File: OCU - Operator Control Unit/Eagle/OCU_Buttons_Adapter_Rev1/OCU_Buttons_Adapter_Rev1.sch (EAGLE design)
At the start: 10 parts, among them J1 1053091202, J2 1053091202, J3 1053091202, J4 1053091202, J5 505567-0271, J6 505567-0271, J7 505567-0371

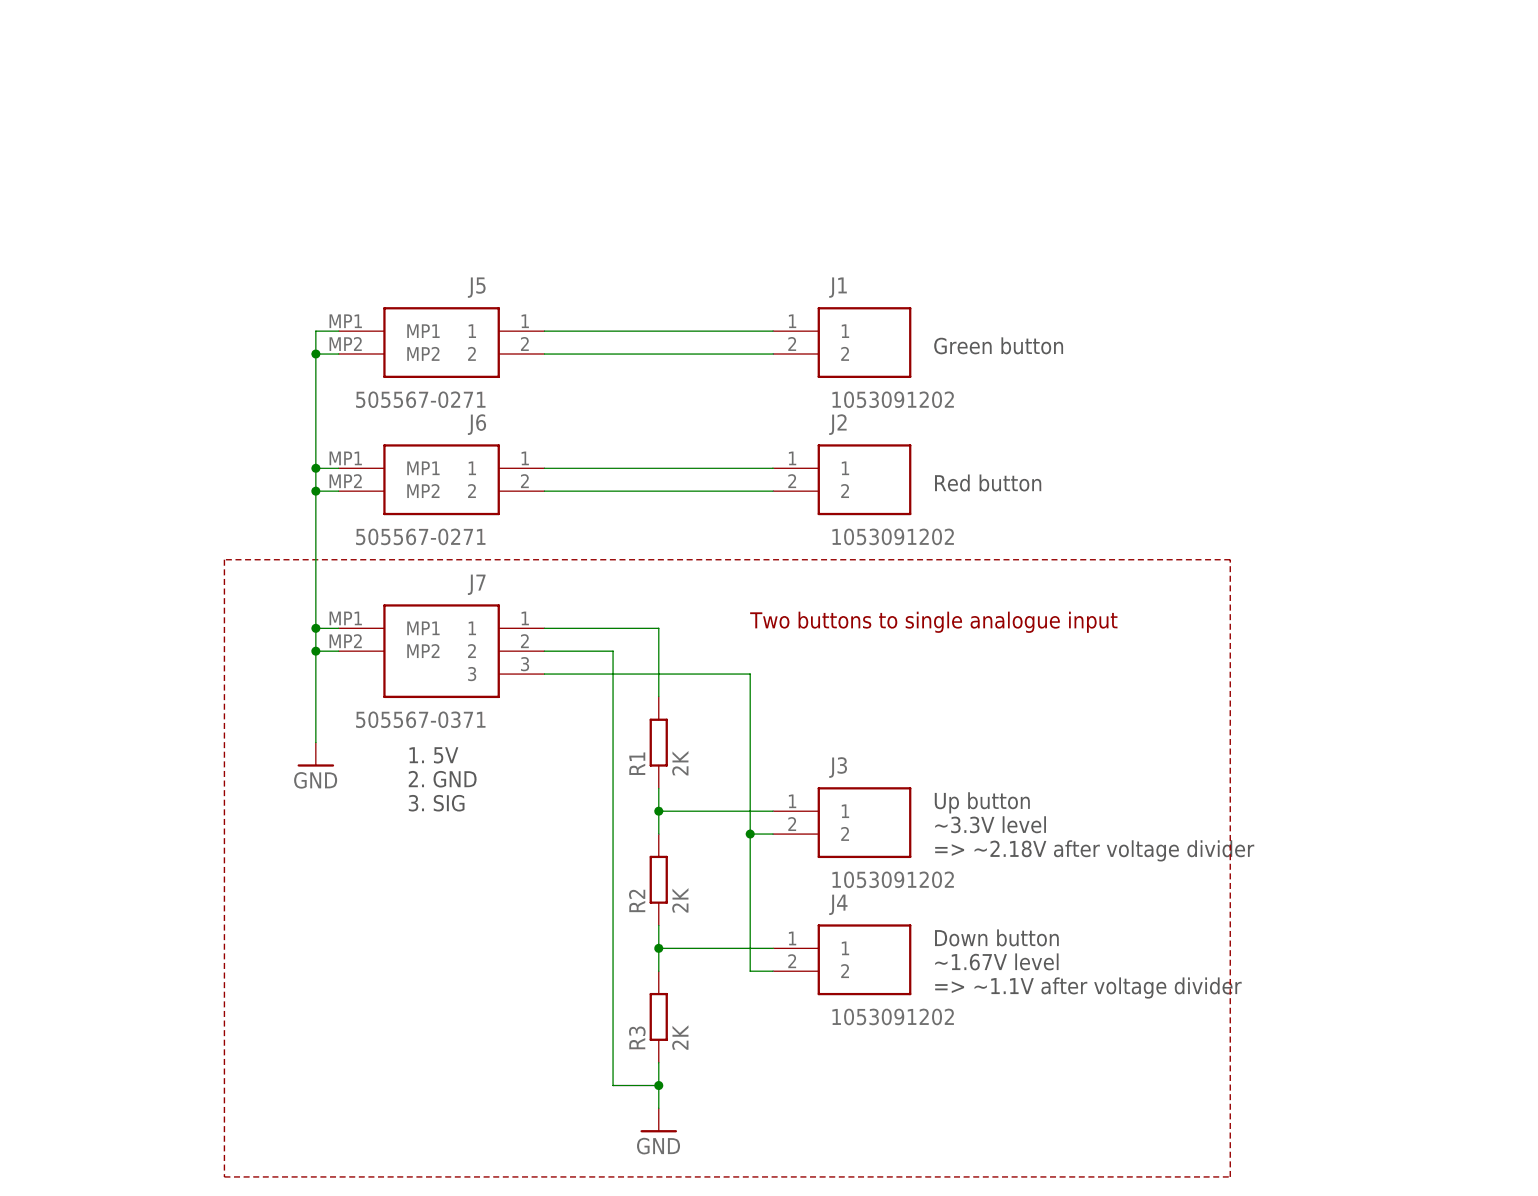
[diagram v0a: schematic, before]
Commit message: -
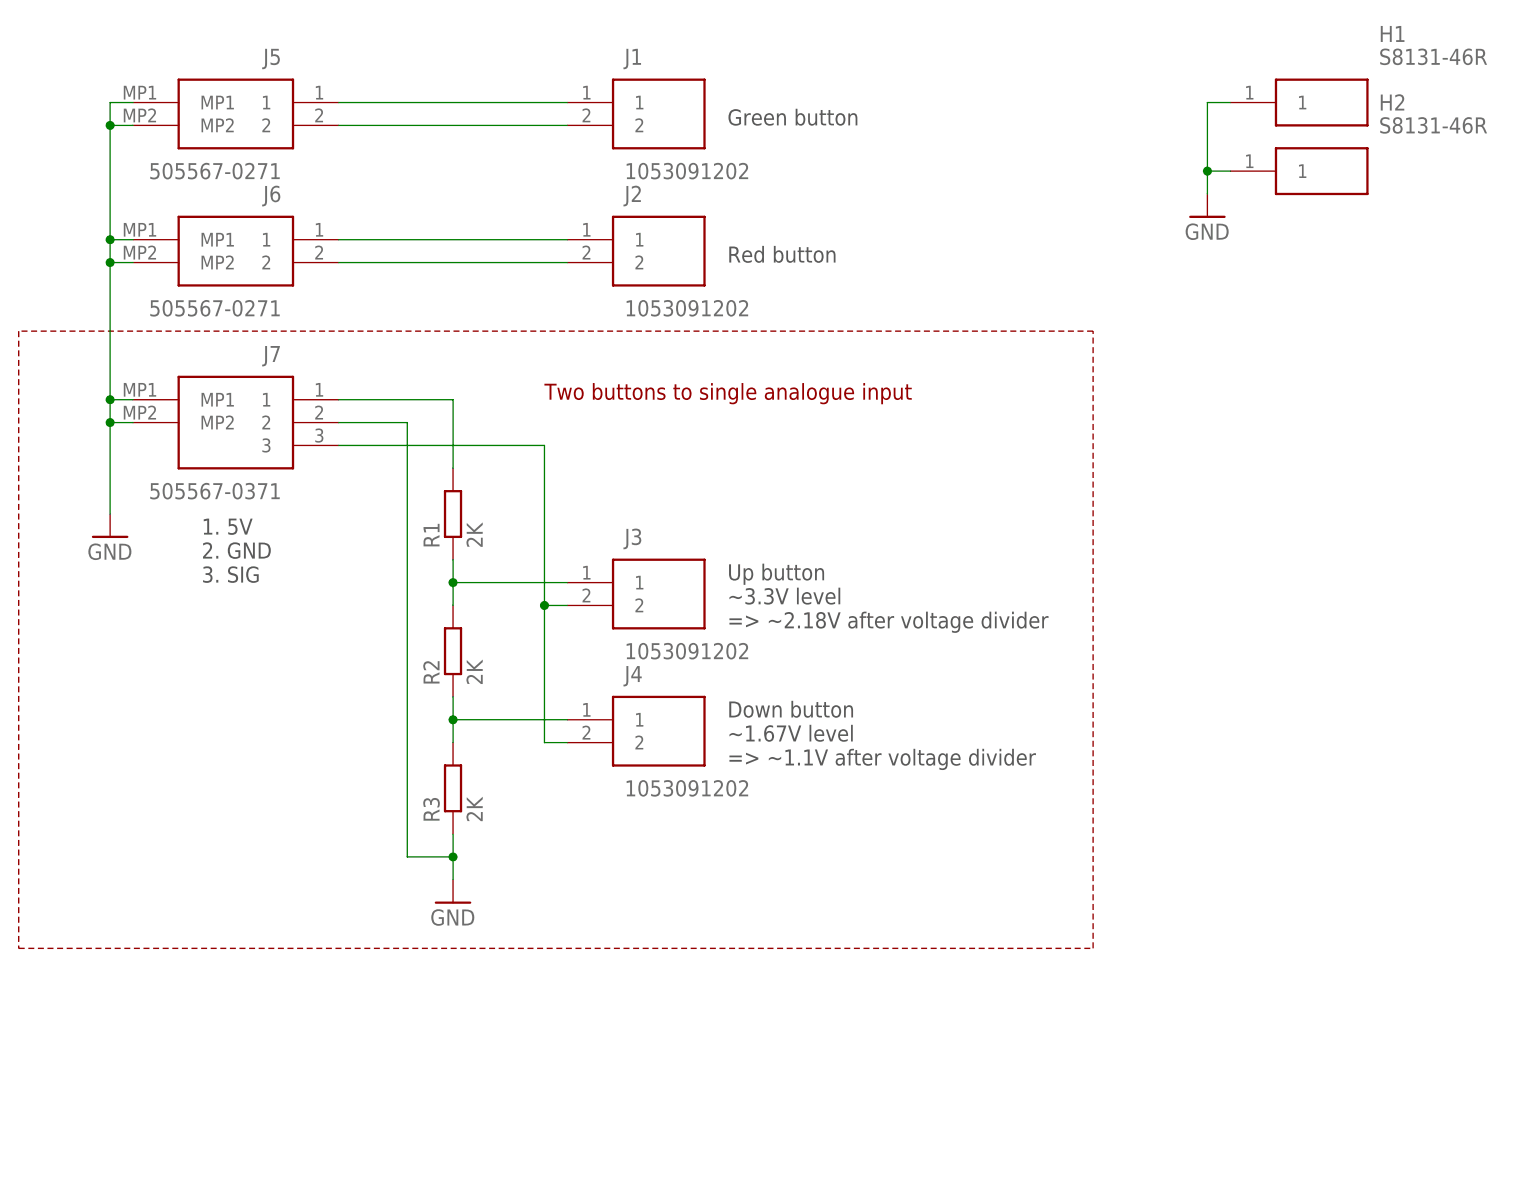
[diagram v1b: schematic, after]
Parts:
- added H1, H2: S8131-46R, RescueRunner:S8131-46R
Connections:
- net GND: now also H1.1, H2.1
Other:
- moved on the sheet: J1, J2, J3, J4, J5, J6, J7, R1, R2, R3
